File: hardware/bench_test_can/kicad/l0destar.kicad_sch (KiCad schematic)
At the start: 7 parts, among them J2 Conn_01x12_Socket, J4 Conn_01x18_Socket

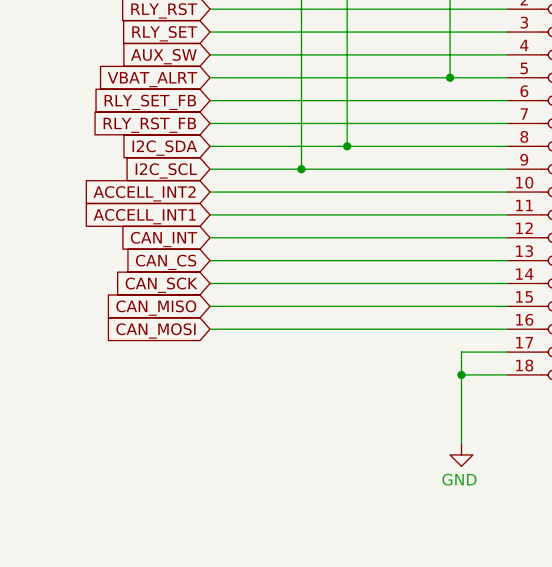
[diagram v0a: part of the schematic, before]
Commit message: fix date
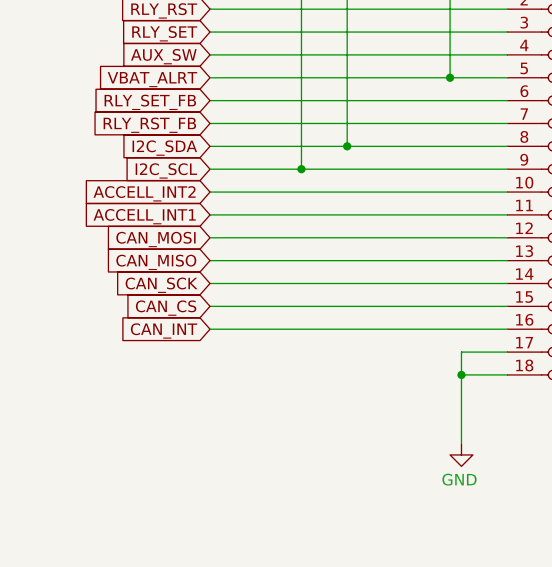
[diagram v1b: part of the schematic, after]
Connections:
- net CAN_CS: now also J4.15 (Pin_15); no longer J4.13 (Pin_13)
- net CAN_INT: now also J4.16 (Pin_16); no longer J4.12 (Pin_12)
- net CAN_MISO: now also J4.13 (Pin_13); no longer J4.15 (Pin_15)
- net CAN_MOSI: now also J4.12 (Pin_12); no longer J4.16 (Pin_16)
